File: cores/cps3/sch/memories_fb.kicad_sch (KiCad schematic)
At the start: 4 parts

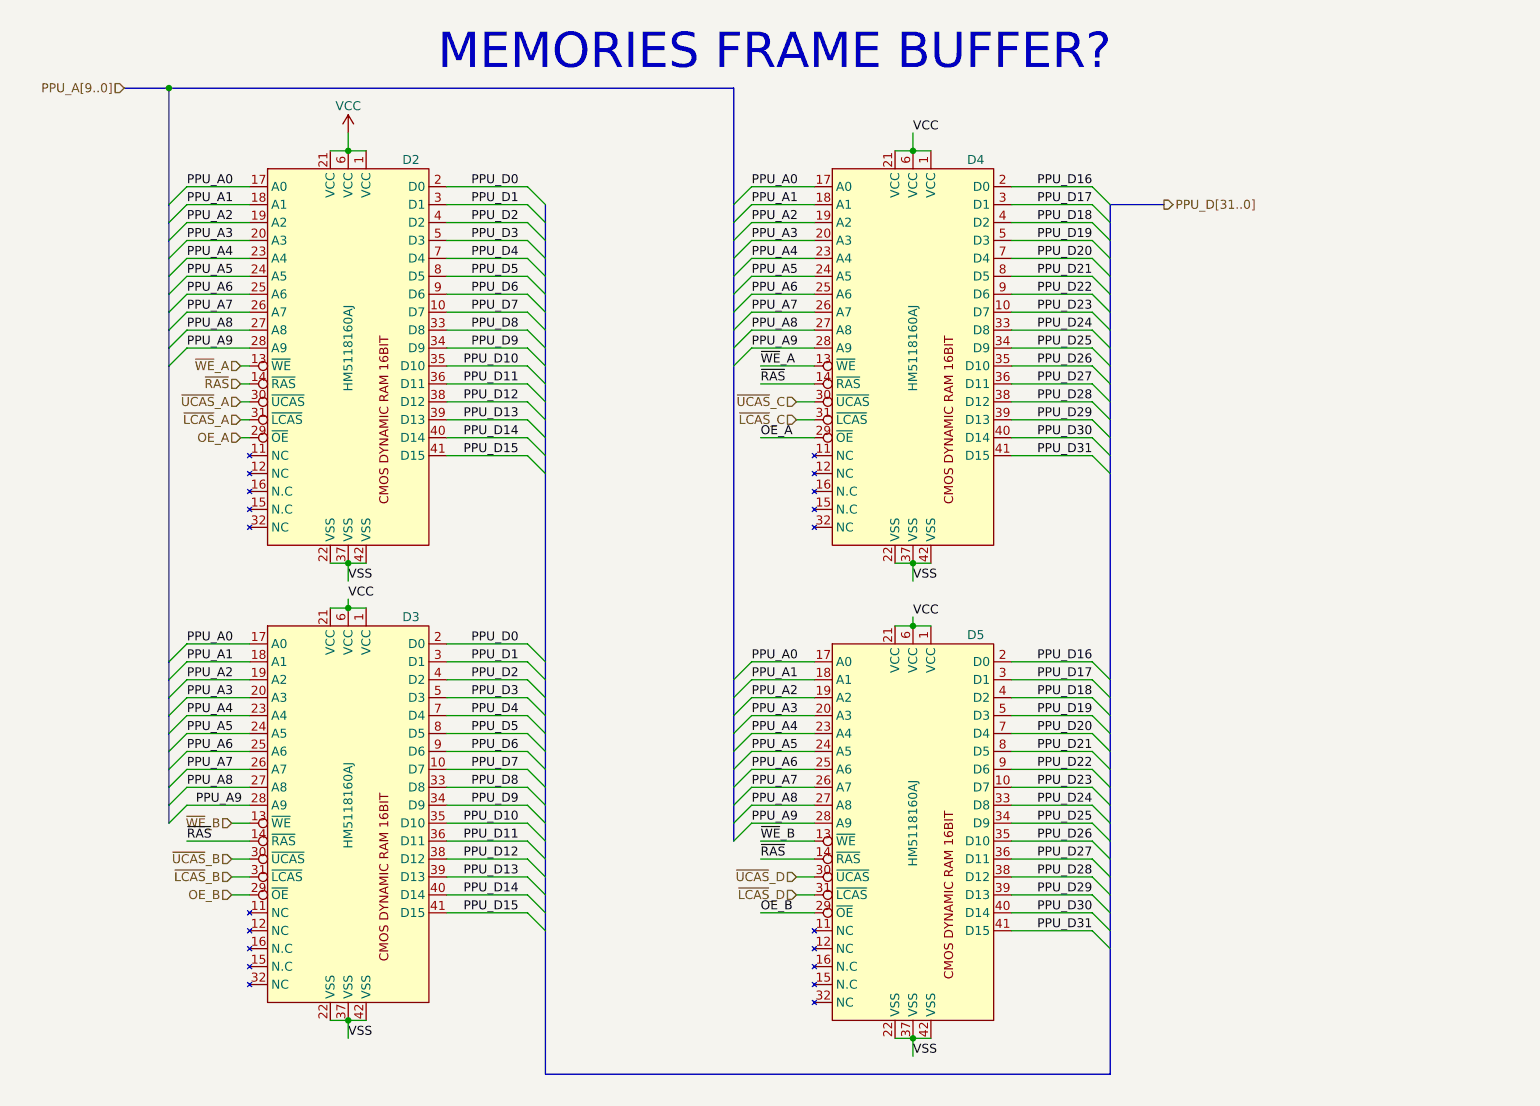
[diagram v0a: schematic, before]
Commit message: wip_ccu
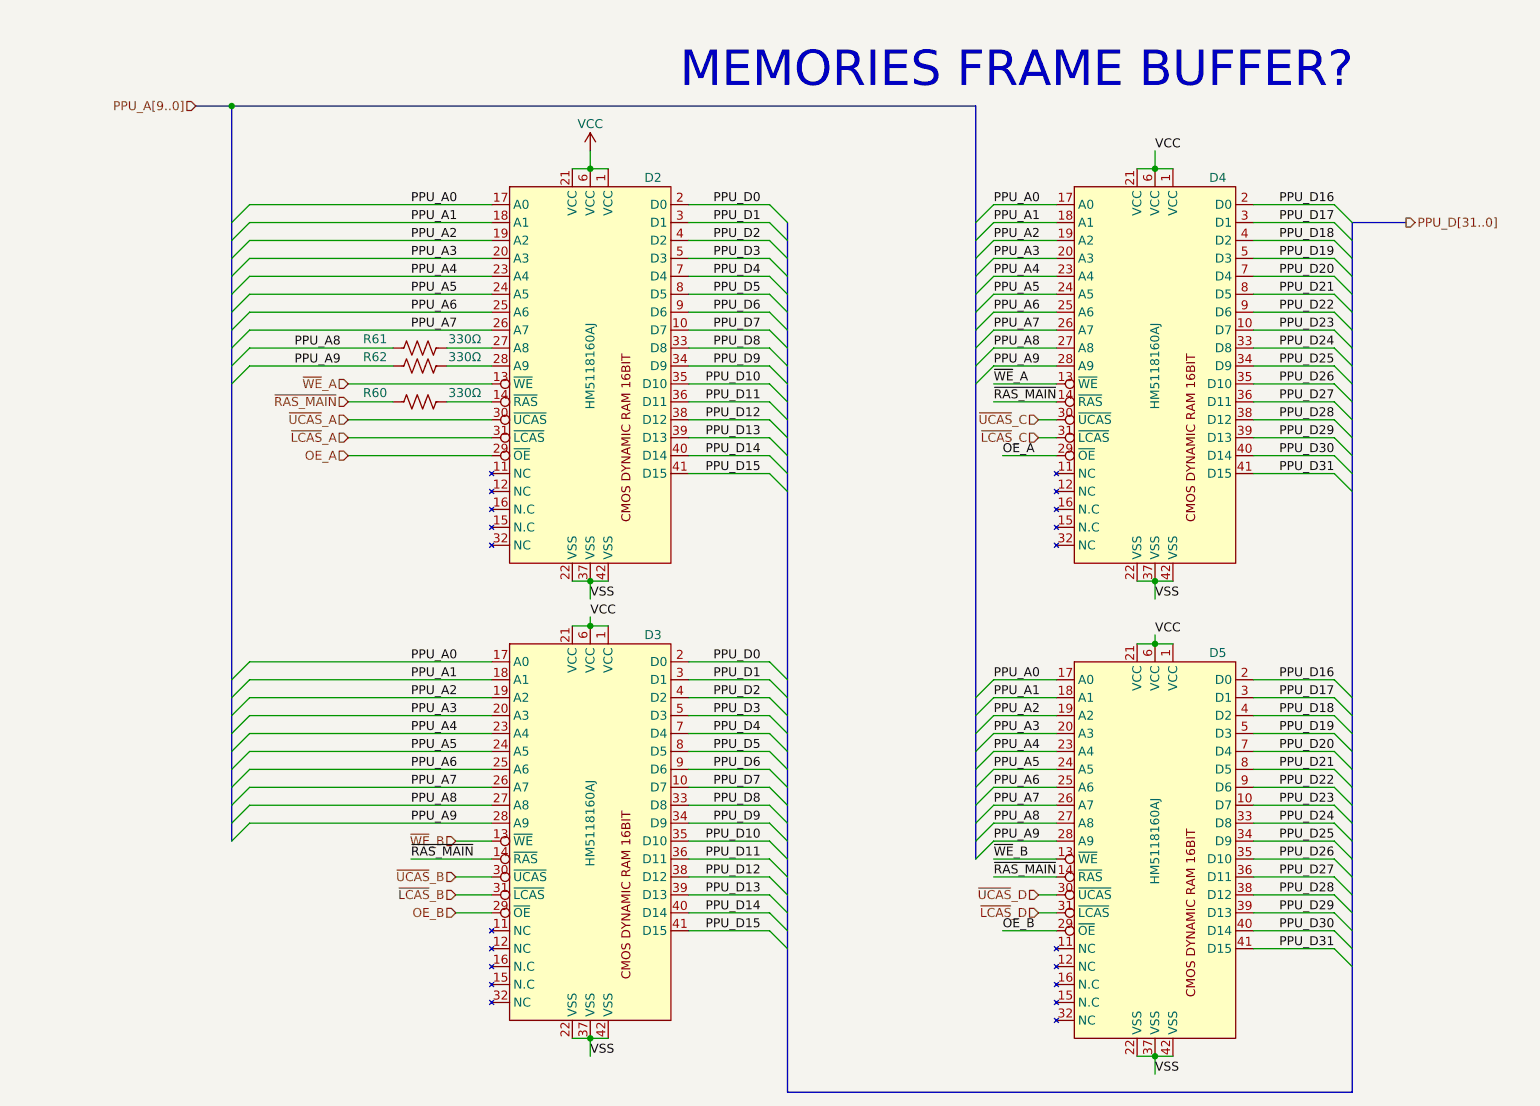
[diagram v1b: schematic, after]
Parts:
- added R60, R61, R62: 330Ω, symbol Device:R_US
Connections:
- net PPU_A8: now also R61.1; no longer D2.27 (A8)
- net PPU_A9: now also R62.1; no longer D2.28 (A9)
- net ~{RAS} renamed ~{RAS_MAIN}
- net ~{RAS_MAIN}: now also R60.1; no longer D2.14 (~{RAS})
- new net: D2.28 (A9), R62.2
- new net: D2.14 (~{RAS}), R60.2
- new net: D2.27 (A8), R61.2
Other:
- moved on the sheet: D2, D3, D4, D5
